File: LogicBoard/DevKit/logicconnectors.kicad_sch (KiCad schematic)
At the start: 28 parts, among them J1 ServoConn, J1 USBC Socket, J10 PhaseConn1, J11 SPI1Conn, J12 UART2Conn, J18 PhaseConn1, J19 PhaseConn1, J2 AuxConn, J20 SPI1Conn, J22 UART3Conn, J5 HallConn, J6 UARTConn, J7 JTAG, J8 CANConn, U6 TJA1050T/CM,118, U7 USBLC6-2SC6

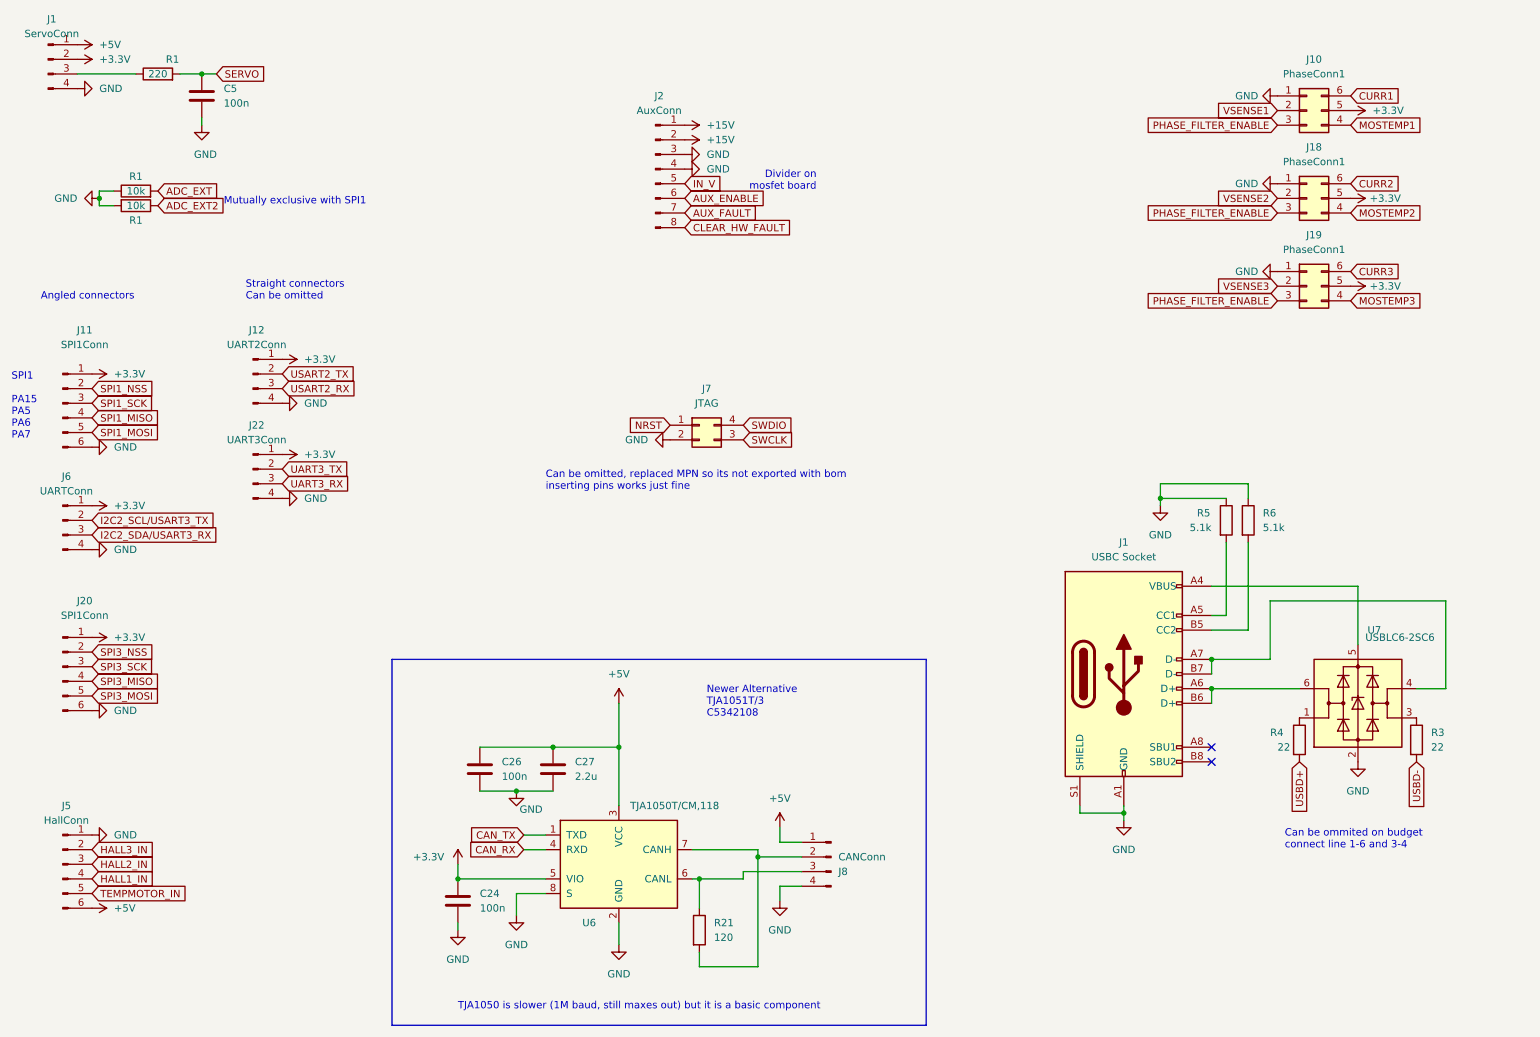
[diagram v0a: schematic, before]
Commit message: v2.3
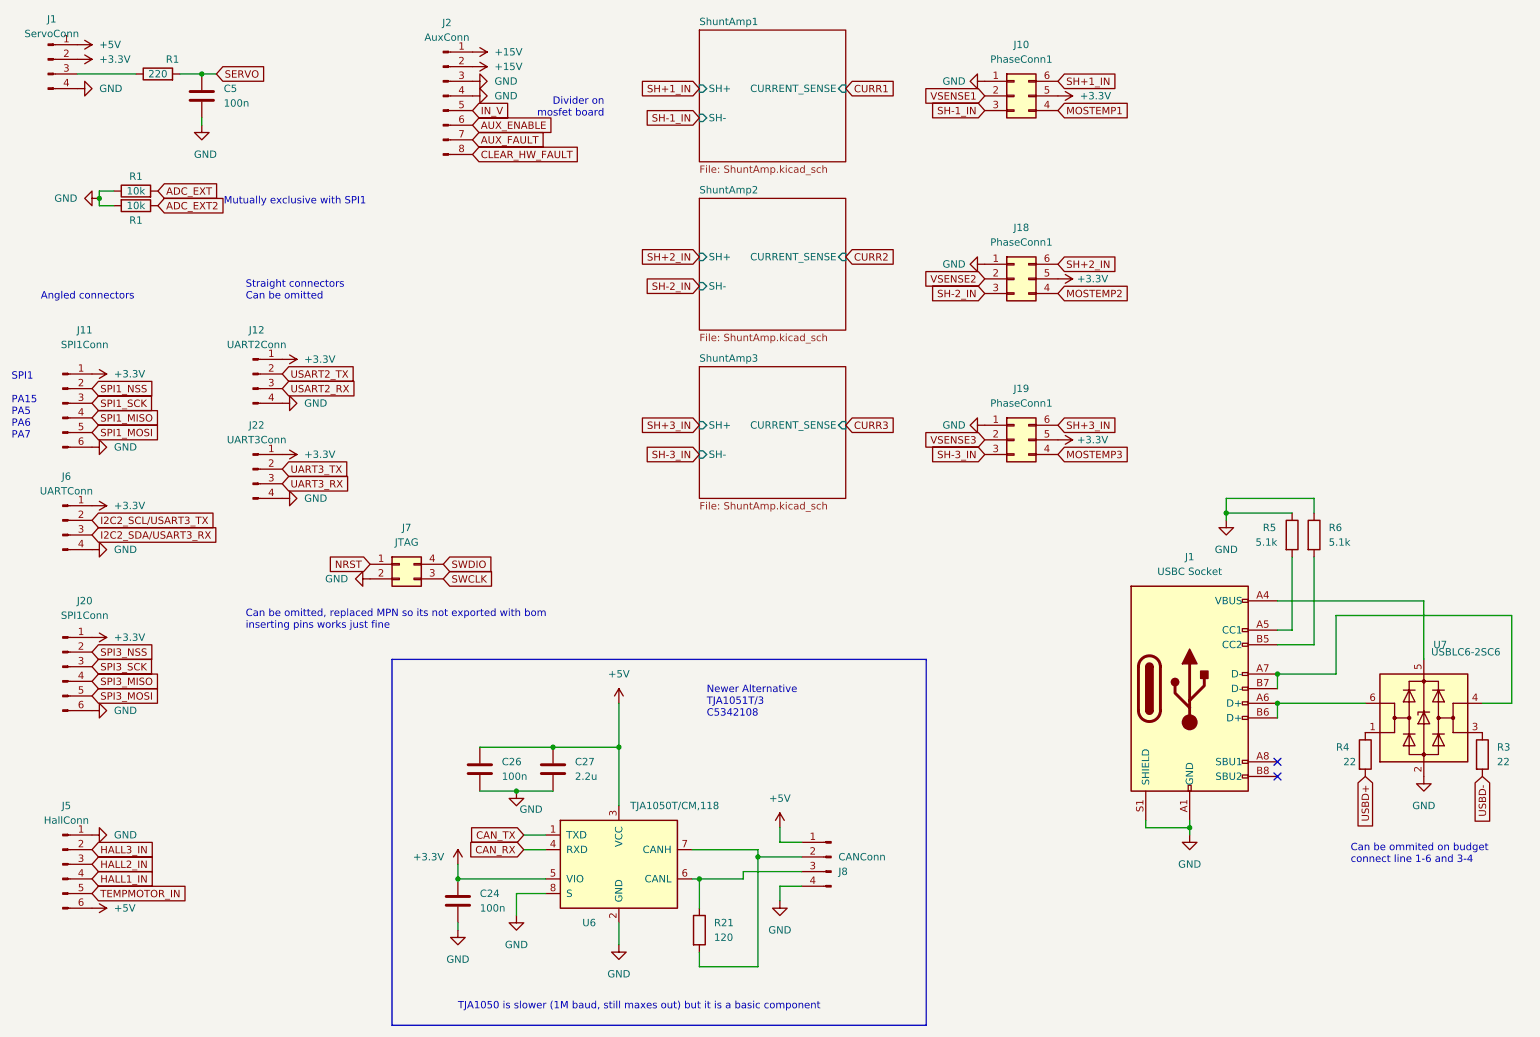
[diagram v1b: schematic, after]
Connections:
- net CURR1: no longer J10.6 (Pin_6)
- net CURR2: no longer J18.6 (Pin_6)
- net CURR3: no longer J19.6 (Pin_6)
- removed net PHASE_FILTER_ENABLE: J10.3 (Pin_3), J18.3 (Pin_3), J19.3 (Pin_3)
- new net SH+1_IN: J10.6 (Pin_6)
- new net SH+2_IN: J18.6 (Pin_6)
- new net SH+3_IN: J19.6 (Pin_6)
- new net SH-1_IN: J10.3 (Pin_3)
- new net SH-2_IN: J18.3 (Pin_3)
- new net SH-3_IN: J19.3 (Pin_3)
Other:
- added sheet ShuntAmp1 (ShuntAmp.kicad_sch)
- added sheet ShuntAmp2 (ShuntAmp.kicad_sch)
- added sheet ShuntAmp3 (ShuntAmp.kicad_sch)
- moved on the sheet: J1, J10, J18, J19, J2, J7, R3, R4, R5, R6, U7
